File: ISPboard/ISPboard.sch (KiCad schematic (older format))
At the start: 17 parts, among them IC1 ATMEGA328-P, P1 5V, P2 ISP, P3 PB, P4 PC, P5 PD, P6 LED OUT, P7 BUTTON OUT, SW1 PUSH 1, SW2 PUSH 2

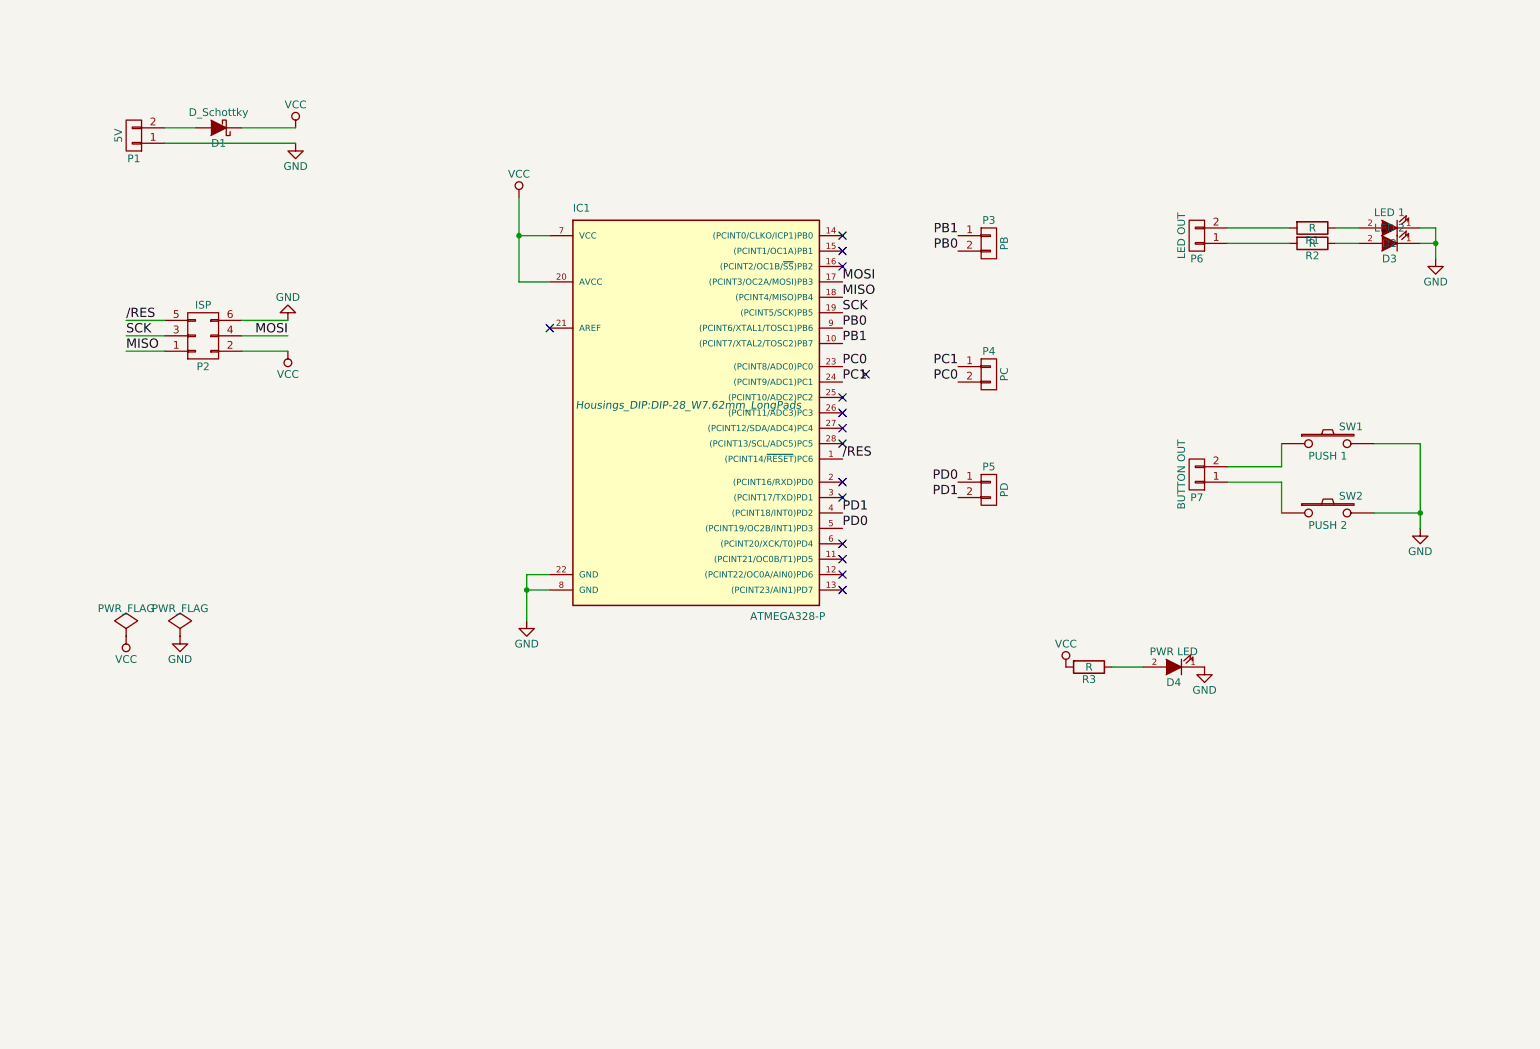
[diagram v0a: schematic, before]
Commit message: Added the avr alarm project
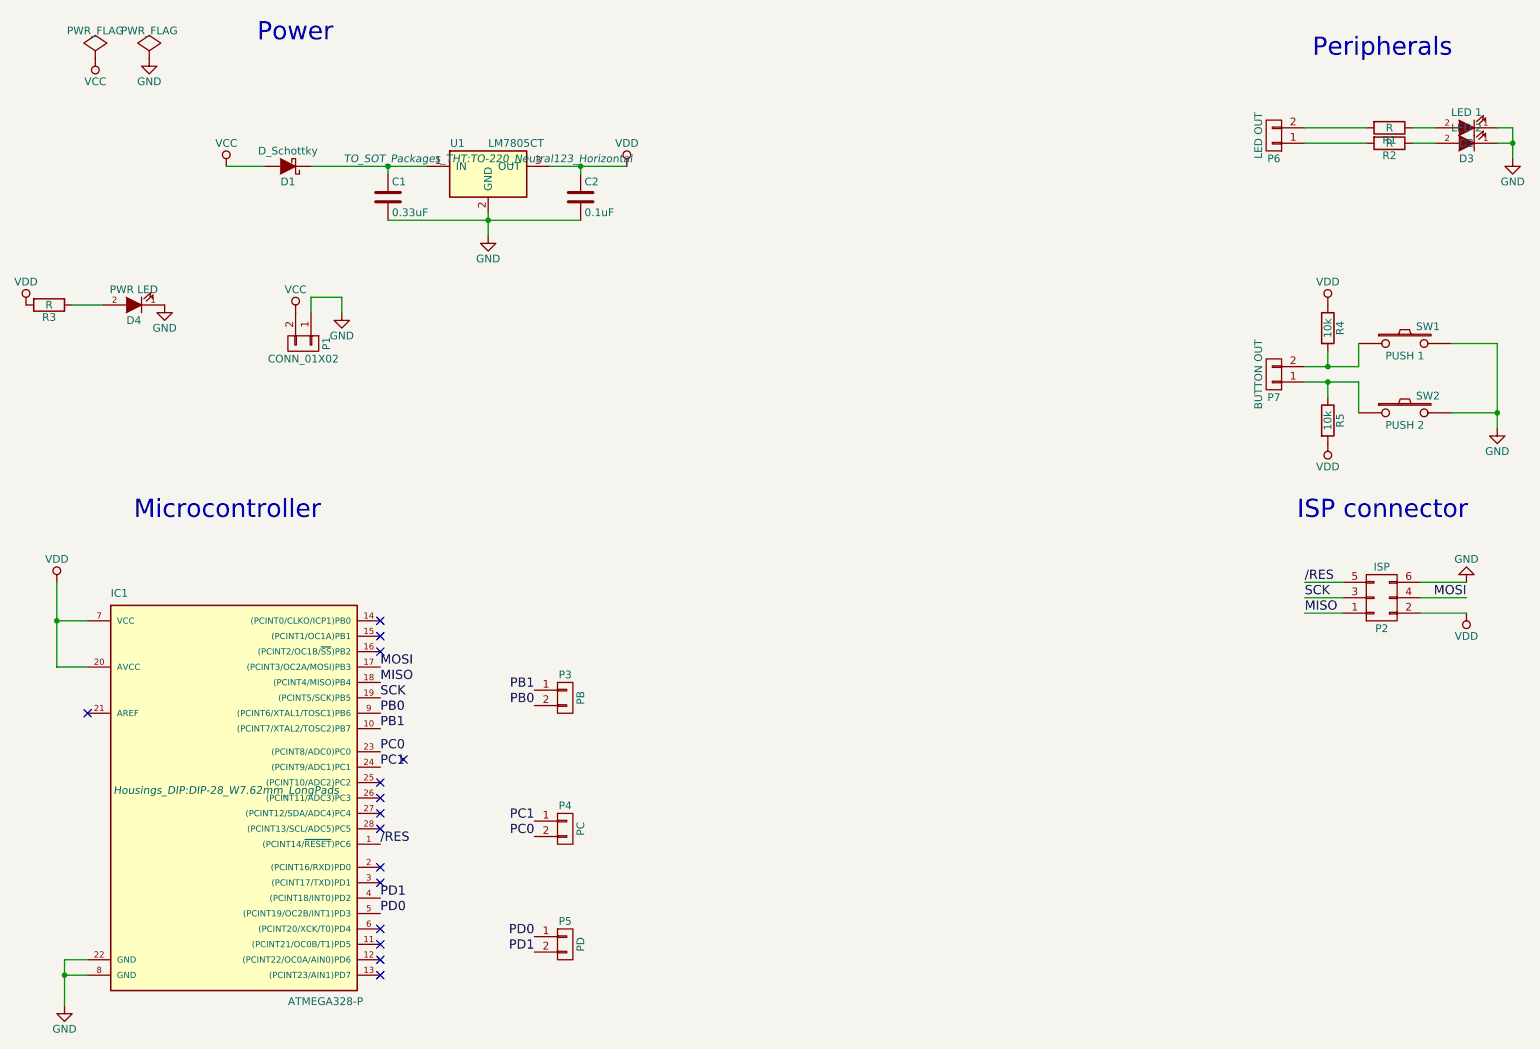
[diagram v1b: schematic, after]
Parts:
- added C1: 0.33uF, Capacitors_ThroughHole:C_Radial_D10_L20_P5, symbol C
- added C2: 0.1uF, Capacitors_ThroughHole:C_Radial_D10_L20_P7.5, symbol C
- added R4, R5: 10k, Resistors_ThroughHole:Resistor_Vertical_RM5mm, symbol R
- added U1: LM7805CT, TO_SOT_Packages_THT:TO-220_Neutral123_Horizontal, symbol LM7805CT
- P1: value 5V -> CONN_01X02
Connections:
- net GND: now also C1.2, C2.2, U1.2 (GND)
- net VCC: now also D1.2 (A), P1.2 (P2); no longer D1.1 (K), IC1.20 (AVCC), IC1.7 (VCC), P2.2 (P2), R3.2
- net at P7.1 (P1), SW2.1: now also R5.1
- net at P7.2 (P2), SW1.1: now also R4.2
- new net: C1.1, D1.1 (K), U1.1 (IN)
- new net VDD: C2.1, IC1.20 (AVCC), IC1.7 (VCC), P2.2 (P2), R3.2, R4.1, R5.2, U1.3 (OUT)
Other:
- note added: "ISP connector"
- note added: "Microcontroller"
- note added: "Peripherals"
- note added: "Power"
- moved on the sheet: D2, D3, D4, IC1, P2, P3, P4, P5, P6, P7, R1, R2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
